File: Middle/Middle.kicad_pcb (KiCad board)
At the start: 2 copper layers, 130 parts, among them J1 Conn_Ext_4, J10 Conn_01x03_Female, J11 Conn_01x03_Female, J12 Conn_01x03_Female, J13 Conn_01x03_Female, J14 Conn_01x03_Female, J15 Conn_01x03_Female, J16 Conn_01x03_Female, J17 Conn_01x03_Female, J18 Conn_01x03_Female, J19 Conn_01x03_Female, J2 Conn_Alt_4, J20 Conn_01x03_Female, J21 Conn_01x03_Female, J22 Conn_01x03_Female, J23 Conn_01x03_Female, J24 Conn_01x03_Female, J25 Conn_01x03_Female, J26 Conn_Ext_8, J27 SWD_TAG_Connector, J28 Conn_Alt_8, J29 Conn_Ext_4, J3 Conn_Ext_4, J30 Conn_Alt_4, J31 Conn_Ext_4, J32 Conn_Alt_4, J4 Conn_Alt_4, J5 Conn_Ext_8, J6 Conn_SWD, J7 Conn_Alt_8, J8 Conn_01x03_Female, J9 Conn_01x03_Female, Q1 NMOS, Q10 NMOS, Q11 NMOS, Q12 NMOS, Q2 NMOS, Q3 NMOS, Q4 NMOS, Q5 NMOS, Q6 NMOS, Q7 NMOS, Q8 NMOS, Q9 NMOS, SW1 SW_Push, U1 TLVM23625RDNR, U2 STM32G070KBT6, U3 AP7361C-33E, U4 TXB0102DCU, U5 SN74LV4052APW, Y1 Crystal_GND24

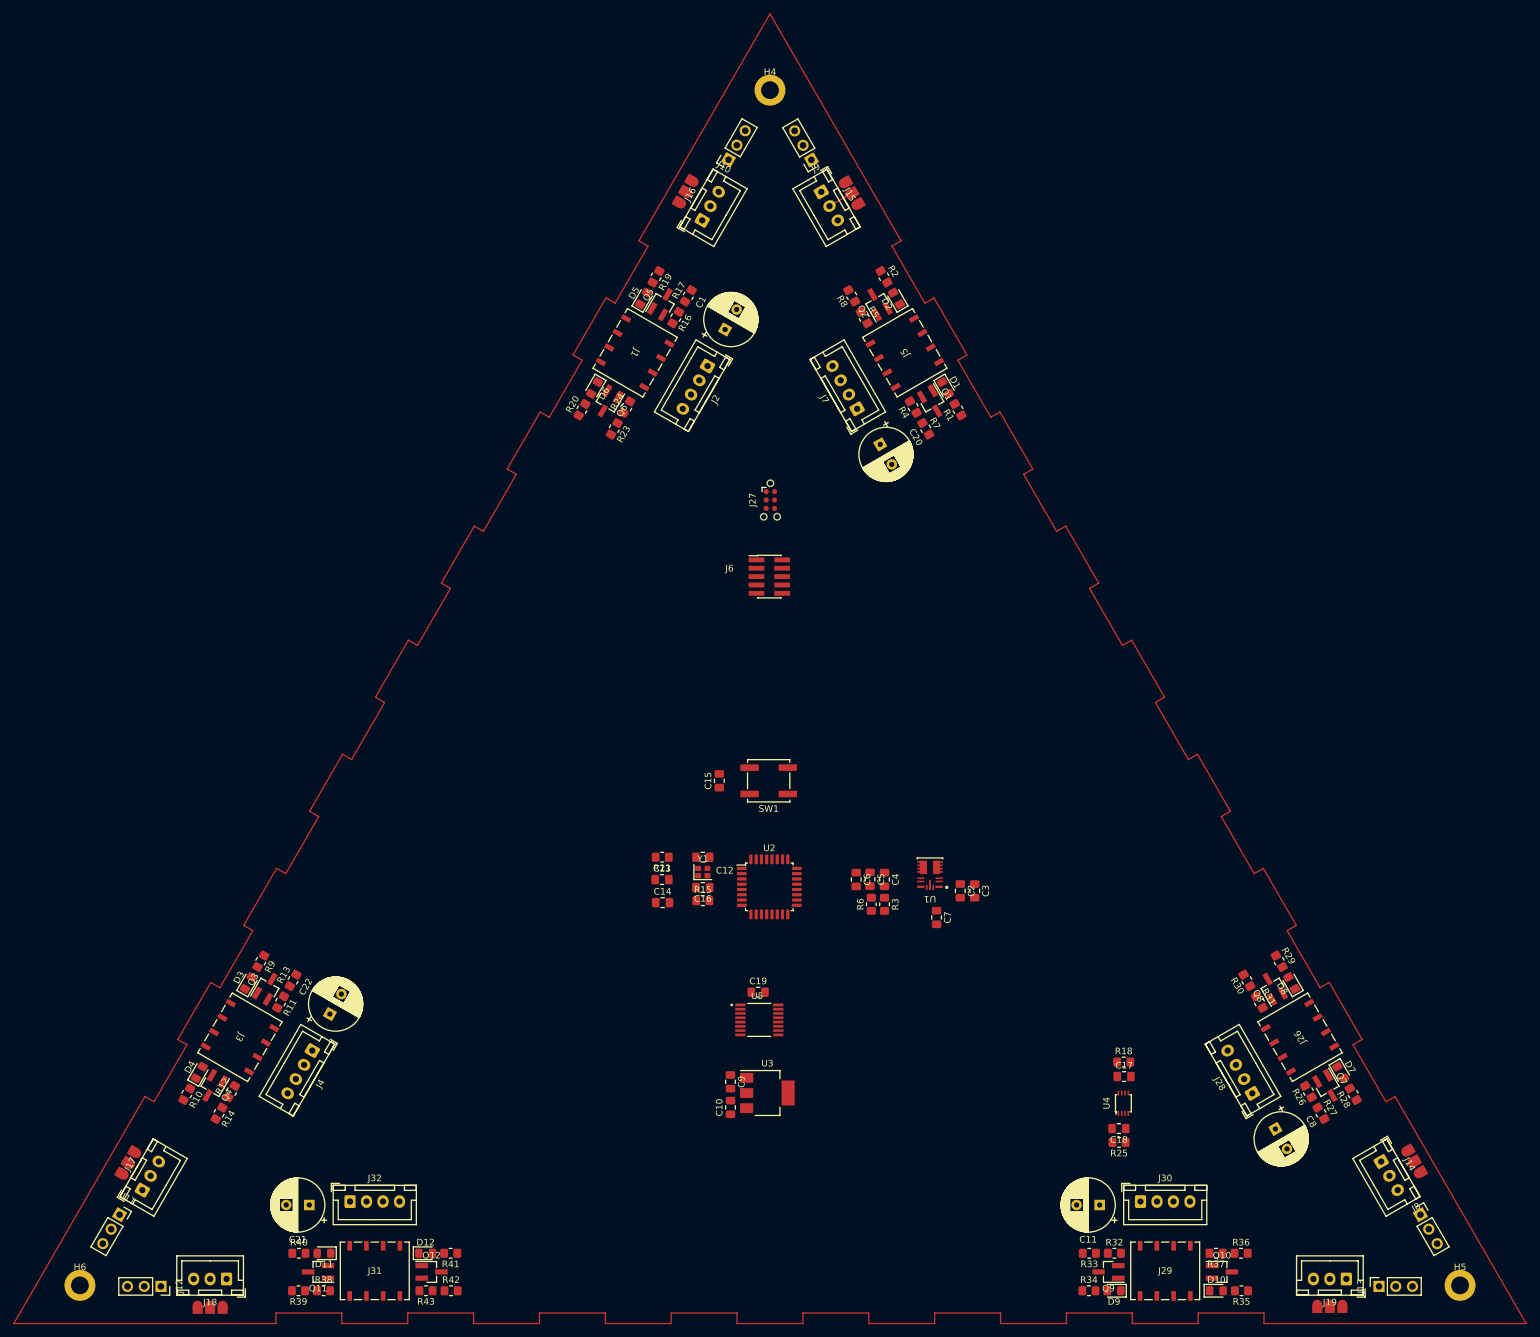
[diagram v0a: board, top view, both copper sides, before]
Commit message: MiddleSize Nanoleaf Finished
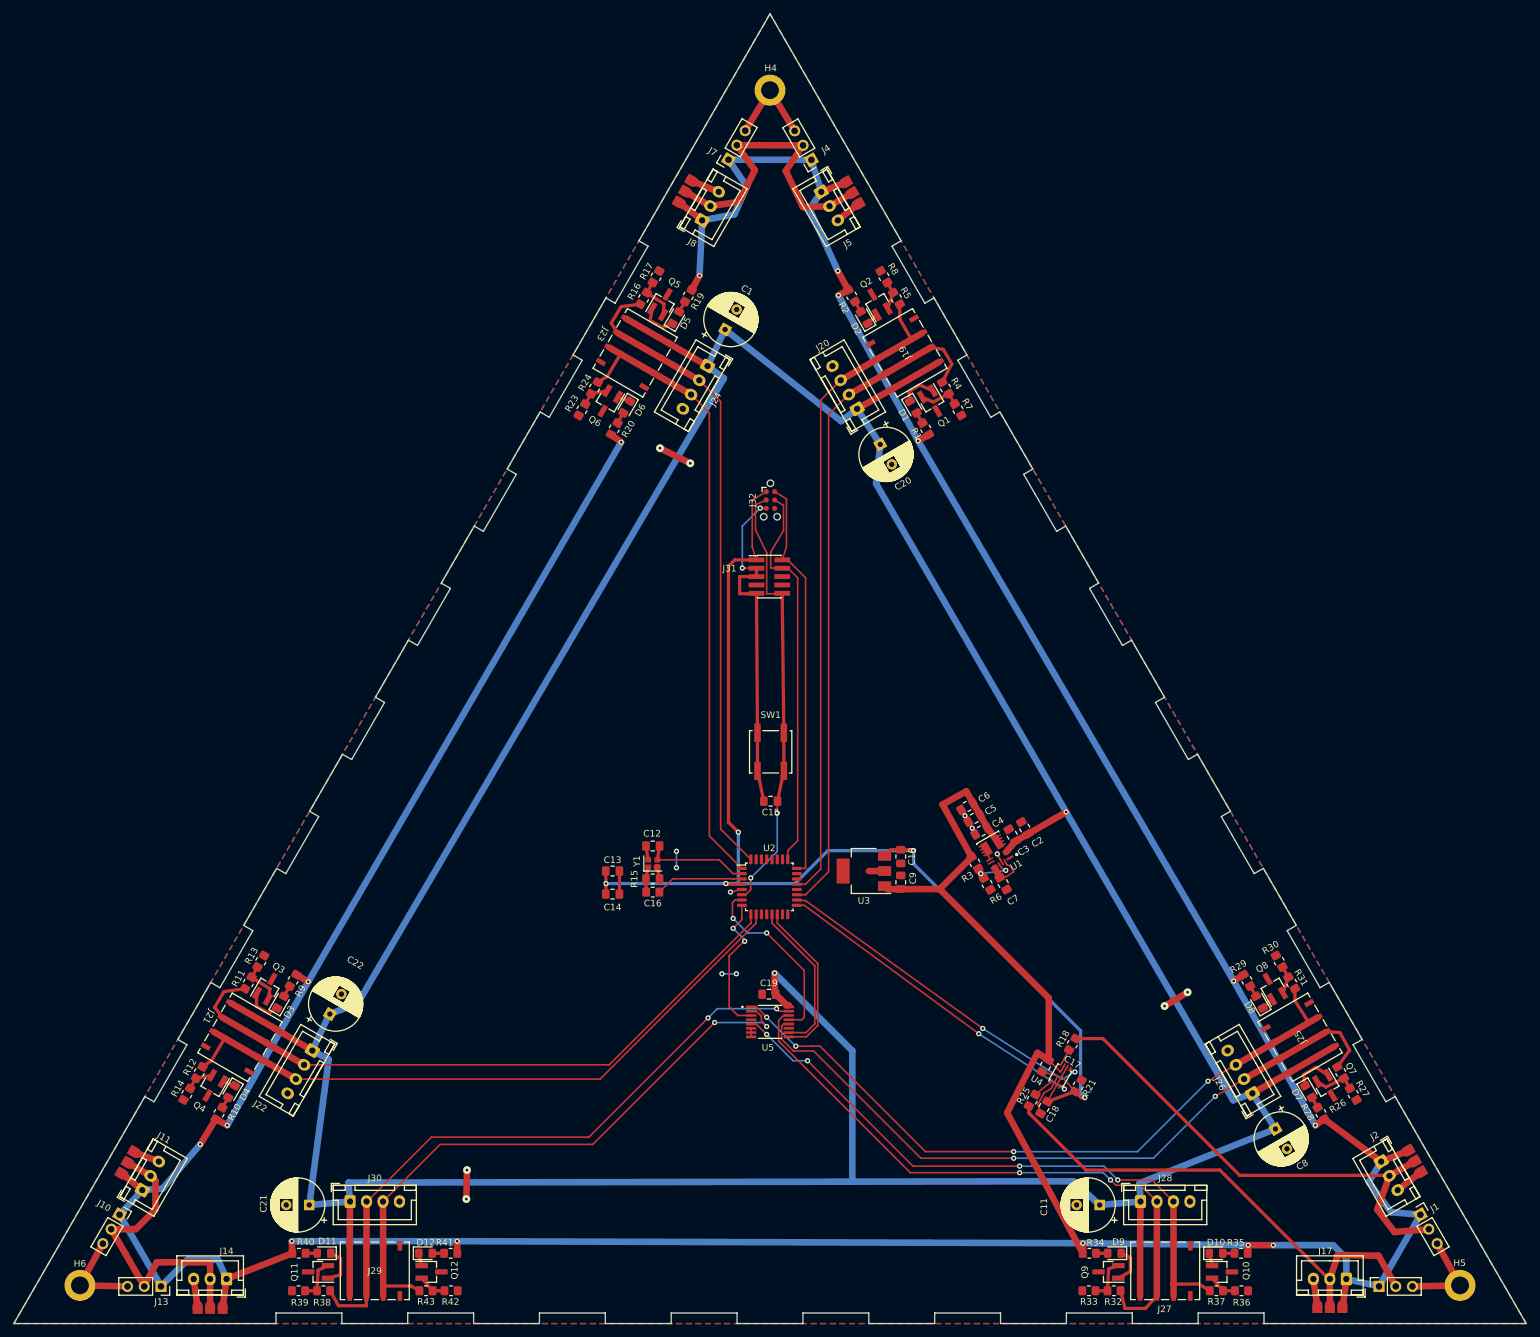
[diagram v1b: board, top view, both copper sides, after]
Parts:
- D8: value LED -> locked
- moved R21 72.1 mm to (191.4, 223.8), turned to -120 degrees
- moved C10 46.0 mm to (164.4, 189.0), turned to -90 degrees
- moved C9 39.8 mm to (164.4, 192.9), turned to 90 degrees
- moved U3 36.7 mm to (158.8, 191.2), turned to 180 degrees
- moved C6 20.2 mm to (174.5, 181.4), turned to -150 degrees
- moved C5 18.3 mm to (175.6, 183.2), turned to -150 degrees
- moved R6 17.8 mm to (177.6, 193.2), turned to -60 degrees
- moved C4 16.4 mm to (176.7, 185.1), turned to -150 degrees
- moved R3 15.1 mm to (175.7, 190.0), turned to -60 degrees
- moved R25 14.7 mm to (184.4, 226.0), turned to 60 degrees
- moved C2 13.7 mm to (183.3, 184.7), turned to 120 degrees
- moved C17 12.1 mm to (186.4, 220.8), turned to -120 degrees
- moved C18 11.8 mm to (186.2, 227.1), turned to -120 degrees
- moved C7 11.3 mm to (180.0, 193.1), turned to -60 degrees
- moved U1 10.5 mm to (178.8, 188.2), turned to -150 degrees
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- renumbered J8 to J1, J11 to J10, J17 to J11, J23 to J12, J12 to J13, J18 to J14, J24 to J15, J13 to J16, J19 to J17, J25 to J18, J5 to J19, J14 to J2, J7 to J20, J3 to J21, J4 to J22, J1 to J23, J2 to J24, J26 to J25, J28 to J26, J29 to J27, J30 to J28, J31 to J29, J20 to J3, J32 to J30, J6 to J31, J27 to J32, J9 to J4, J15 to J5, J21 to J6, J10 to J7, J16 to J8, J22 to J9
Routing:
- net +5V: track 0.00 -> 745.4 mm, vias 0 -> 15
- net VDD: track 0.00 -> 606.4 mm, vias 0 -> 2
- net +3V3: track 0.00 -> 188.4 mm, vias 0 -> 5
- net GND: track 0.00 -> 168.5 mm, vias 0 -> 16
- net /UART_4_TX: track 0.00 -> 108.2 mm, vias 0 -> 2
- net /UART_4_RX: track 0.00 -> 107.9 mm, vias 0 -> 4
- net /UART_1_TX: track 0.00 -> 102.0 mm
- net /UART_2_RX: track 0.00 -> 101.0 mm
- net /UART_2_TX: track 0.00 -> 100.3 mm
- net /UART_1_RX: track 0.00 -> 100.2 mm
- net /UART_6_TX: track 0.00 -> 99.0 mm, vias 0 -> 2
- net /UART_3_TX: track 0.00 -> 97.9 mm
- net /UART_5_RX: track 0.00 -> 95.4 mm, vias 0 -> 4
- net /UART_5_TX: track 0.00 -> 95.3 mm, vias 0 -> 2
- net /UART_3_RX: track 0.00 -> 95.1 mm
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- added copper zone on B.Cu, net GND
- added copper zone on F.Cu, net GND
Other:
- board outline added: 229.6 x 198.8 mm
